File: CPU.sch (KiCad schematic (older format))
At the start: 4 parts

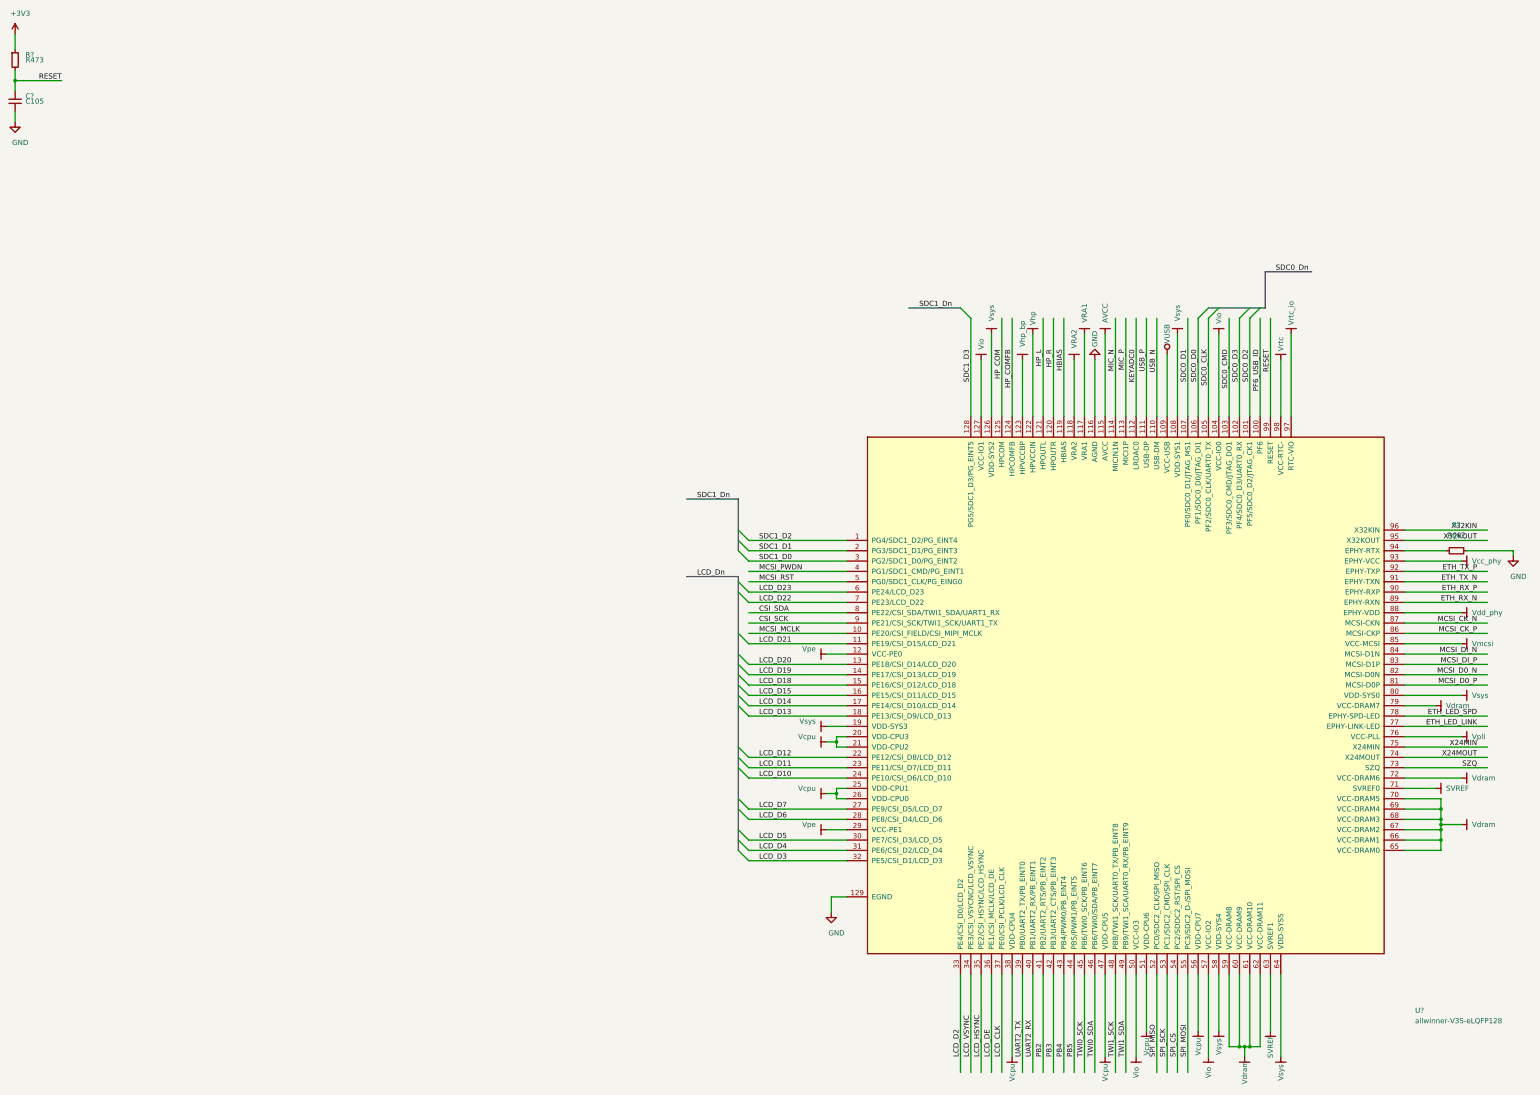
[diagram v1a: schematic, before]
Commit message: update,
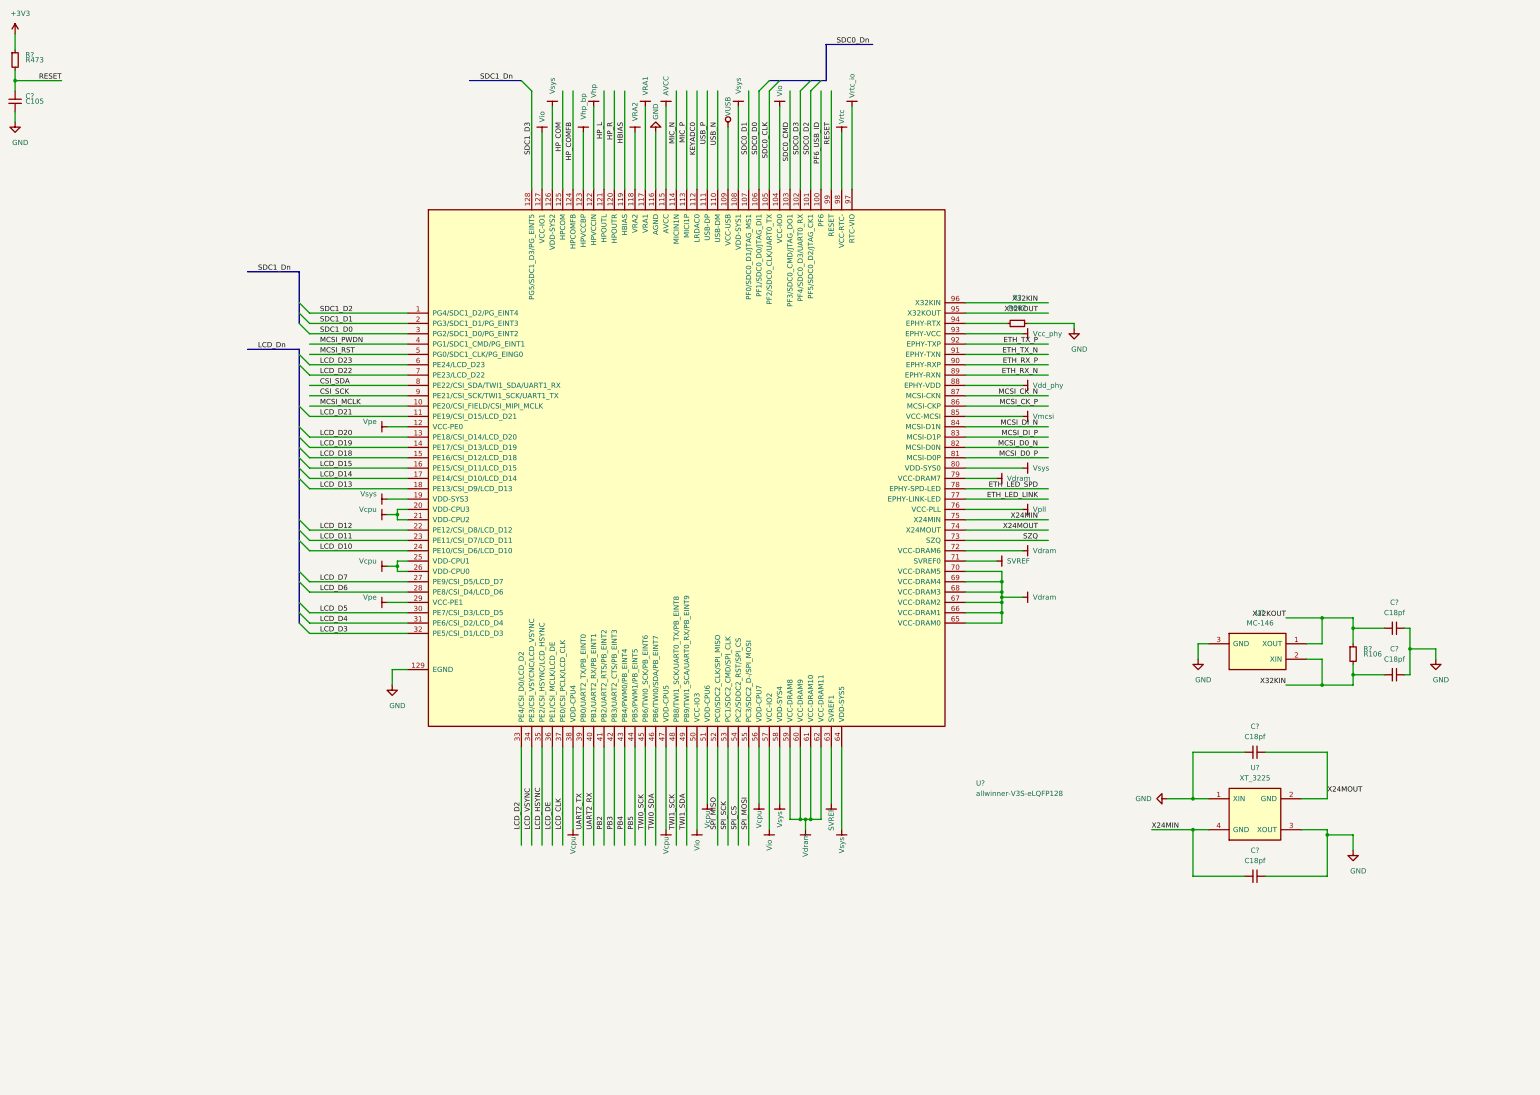
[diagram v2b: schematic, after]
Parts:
- added C? (x4): C18pf, symbol taobao-c:C18pf
- added R?: R106, symbol taobao-r:R106
- added U?: MC-146, symbol taobao-components:MC-146
- added U?: XT_3225, symbol taobao-components:XT_3225
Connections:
- wire segments 155 -> 194
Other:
- moved on the sheet: R?, U?
